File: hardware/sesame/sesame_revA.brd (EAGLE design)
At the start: 22.8 x 44.8 mm, 4 parts, among them Q1 TIP120

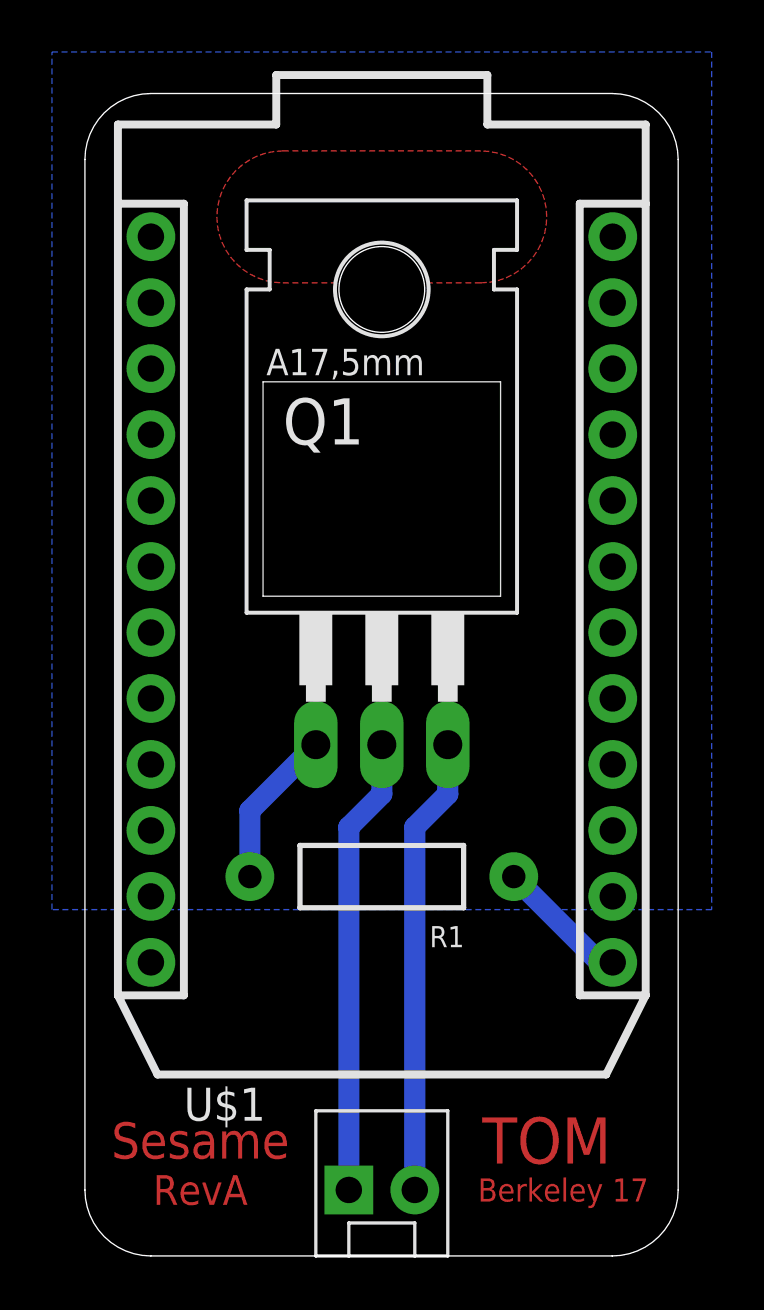
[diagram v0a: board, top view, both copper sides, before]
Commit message: fixing sesame
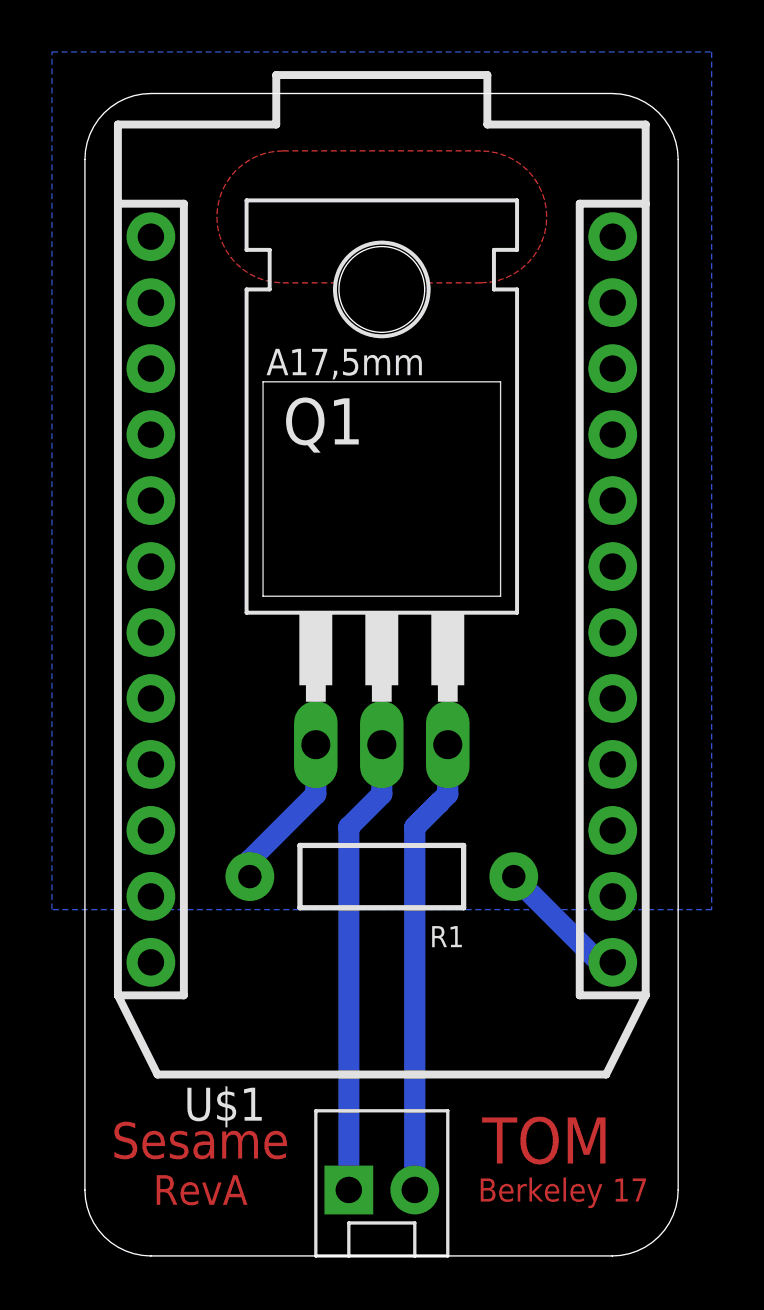
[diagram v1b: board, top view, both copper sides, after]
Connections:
- removed net N$2 (its old number): JP1.2, Q1.E
- net GND: now also JP1.2, Q1.E
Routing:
- net GND: track 0.00 -> 19.0 mm
- net N$2 (its old number): track 17.7 -> 0.00 mm
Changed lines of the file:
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@@
 <vertex x="-1.27" y="7.62"/>
 </polygon>
+<contactref element="Q1" pad="E"/>
+<wire x1="13.97" y1="13.97" x2="13.97" y2="12.065" width="0.8128" layer="16"/>
+<wire x1="13.6525" y1="11.7475" x2="13.97" y2="12.065" width="0.8128" layer="16"/>
+<contactref element="JP1" pad="2"/>
+<wire x1="12.7" y1="10.795" x2="13.6525" y2="11.7475" width="0.8128" layer="16"/>
+<wire x1="12.7" y1="-3.175" x2="12.7" y2="10.795" width="0.8128" layer="16"/>
+<wire x1="12.7" y1="10.795" x2="13.6525" y2="11.7475" width="0.8128" layer="16"/>
 </signal>
 <signal name="3V3">
@@
 <wire x1="11.43" y1="12.065" x2="10.16" y2="10.795" width="0.8128" layer="16"/>
 <wire x1="10.16" y1="10.795" x2="10.16" y2="-3.175" width="0.8128" layer="16"/>
-</signal>
-<signal name="N$2">
-<contactref element="JP1" pad="2"/>
-<contactref element="Q1" pad="E"/>
-<wire x1="13.97" y1="13.97" x2="13.97" y2="12.065" width="0.8128" layer="16"/>
-<wire x1="13.97" y1="12.065" x2="12.7" y2="10.795" width="0.8128" layer="16"/>
-<wire x1="12.7" y1="10.795" x2="12.7" y2="-3.175" width="0.8128" layer="16"/>
-</signal>
-<signal name="N$3">
-<contactref element="Q1" pad="B"/>
-<contactref element="R1" pad="P$2"/>
-<wire x1="6.35" y1="8.89" x2="6.35" y2="11.43" width="0.8128" layer="16"/>
-<wire x1="6.35" y1="11.43" x2="8.89" y2="13.97" width="0.8128" layer="16"/>
 </signal>
 <signal name="N$4">
@@
 </polygon>
 </signal>
+<signal name="N$2">
+<contactref element="R1" pad="P$2"/>
+<contactref element="Q1" pad="B"/>
+<wire x1="8.89" y1="13.97" x2="8.89" y2="12.065" width="0.8128" layer="16"/>
+<wire x1="8.89" y1="12.065" x2="6.35" y2="9.525" width="0.8128" layer="16"/>
+<wire x1="6.35" y1="9.525" x2="6.35" y2="8.89" width="0.8128" layer="16"/>
+</signal>
 </signals>
